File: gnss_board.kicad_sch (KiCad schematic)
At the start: 120 parts, among them J1 Conn_01x10_Pin, J2 Serial Connector, J3 U.FL, J4 Conn_01x04_Pin, Q1 BC817, Q2 BC817, T1 LMUN2211LT1G, U1 H1102NL, U2 LAN8710A, U3 TPS2375D, U4 TX4138(ESOIC-8), U5 ESP32-WROOM-32E, U6 UM980

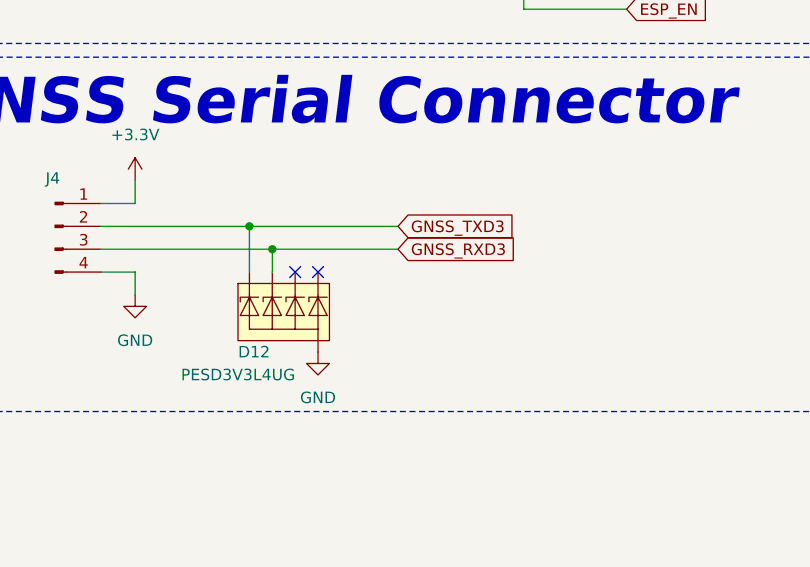
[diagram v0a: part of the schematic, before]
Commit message: Messing around
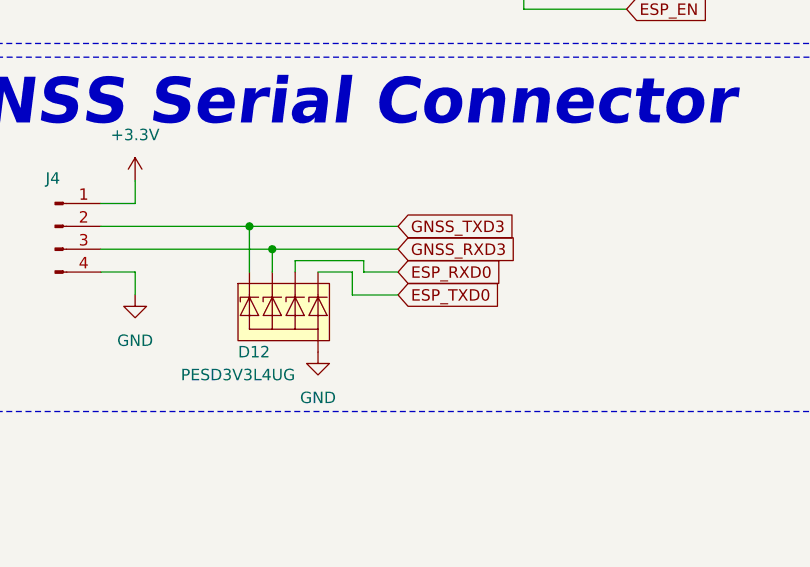
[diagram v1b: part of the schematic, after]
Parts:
- D12: footprint SparkFun-Semiconductor-Standard:SOT-353 -> Package_TO_SOT_SMD:SOT-353_SC-70-5_Handsoldering; PROD_ID DIO-19494 -> (none)
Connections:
- net ESP_RXD0: now also D12.4 (K3)
- net ESP_TXD0: now also D12.5 (K4)
- no-connect marks 36 -> 34
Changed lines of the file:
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@@
 	)
 	(no_connect
-		(at 341.63 234.95)
-	)
-	(no_connect
 		(at 365.76 111.76)
 	)
@@
 	)
 	(no_connect
-		(at 344.17 234.95)
-	)
-	(no_connect
 		(at 233.68 190.5)
 	)
@@
 	(wire
 		(pts
+			(xy 341.63 234.95) (xy 341.63 233.68)
+		)
+		(stroke
+			(width 0)
+			(type default)
+		)
+	)
+	(wire
+		(pts
 			(xy 339.09 232.41) (xy 339.09 234.95)
 		)
@@
 	(wire
 		(pts
+			(xy 347.98 234.95) (xy 347.98 237.49)
+		)
+		(stroke
+			(width 0)
+			(type default)
+		)
+	)
+	(wire
+		(pts
 			(xy 109.22 223.52) (xy 121.92 223.52)
 		)
@@
 	(wire
 		(pts
+			(xy 349.25 233.68) (xy 349.25 234.95)
+		)
+		(stroke
+			(width 0)
+			(type default)
+		)
+	)
+	(wire
+		(pts
 			(xy 46.99 50.8) (xy 46.99 68.58)
 		)
@@
 	(wire
 		(pts
+			(xy 349.25 234.95) (xy 353.06 234.95)
+		)
+		(stroke
+			(width 0)
+			(type default)
+		)
+	)
+	(wire
+		(pts
 			(xy 248.92 106.68) (xy 252.73 106.68)
 		)
@@
 	(wire
 		(pts
+			(xy 344.17 234.95) (xy 347.98 234.95)
+		)
+		(stroke
+			(width 0)
+			(type default)
+		)
+	)
+	(wire
+		(pts
 			(xy 31.75 64.77) (xy 58.42 64.77)
 		)
@@
 	(wire
 		(pts
+			(xy 347.98 237.49) (xy 353.06 237.49)
+		)
+		(stroke
+			(width 0)
+			(type default)
+		)
+	)
+	(wire
+		(pts
 			(xy 214.63 207.01) (xy 214.63 208.28)
 		)
@@
 	(wire
 		(pts
+			(xy 341.63 233.68) (xy 349.25 233.68)
+		)
+		(stroke
+			(width 0)
+			(type default)
+		)
+	)
+	(wire
+		(pts
 			(xy 109.22 226.06) (xy 121.92 226.06)
 		)
@@
 		)
 	)
+	(global_label "ESP_RXD0"
+		(shape input)
+		(at 353.06 234.95 0)
+		(fields_autoplaced yes)
+		(effects
+			(font
+				(size 1.27 1.27)
+			)
+			(justify left)
+		)
+		(property "Intersheetrefs" "${INTERSHEET_REFS}"
+			(at 365.6003 234.95 0)
+			(effects
+				(font
+					(size 1.27 1.27)
+				)
+				(justify left)
+				(hide yes)
+			)
+		)
+	)
 	(global_label "GNSS_RXD2"
 		(shape input)
@@
 		)
 	)
+	(global_label "ESP_TXD0"
+		(shape input)
+		(at 353.06 237.49 0)
+		(fields_autoplaced yes)
+		(effects
+			(font
+				(size 1.27 1.27)
+			)
+			(justify left)
+		)
+		(property "Intersheetrefs" "${INTERSHEET_REFS}"
+			(at 365.2979 237.49 0)
+			(effects
+				(font
+					(size 1.27 1.27)
+				)
+				(justify left)
+				(hide yes)
+			)
+		)
+	)
 	(global_label "ETH_PHY_PWR"
 		(shape input)
@@
 			)
 		)
-		(property "Footprint" "SparkFun-Semiconductor-Standard:SOT-353"
+		(property "Footprint" "Package_TO_SOT_SMD:SOT-353_SC-70-5_Handsoldering"
 			(at 339.09 248.92 0)
 			(effects
@@
 			(effects
 				(font
-					(size 1.27 1.27)
-				)
-				(hide yes)
-			)
-		)
-		(property "PROD_ID" "DIO-19494"
-			(at 339.09 254 0)
-			(effects
-				(font
